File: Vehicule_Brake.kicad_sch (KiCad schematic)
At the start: 22 parts, among them Q51 IRLZ44N, Q53 2N7000, Q54 2N7000, U13 LM339

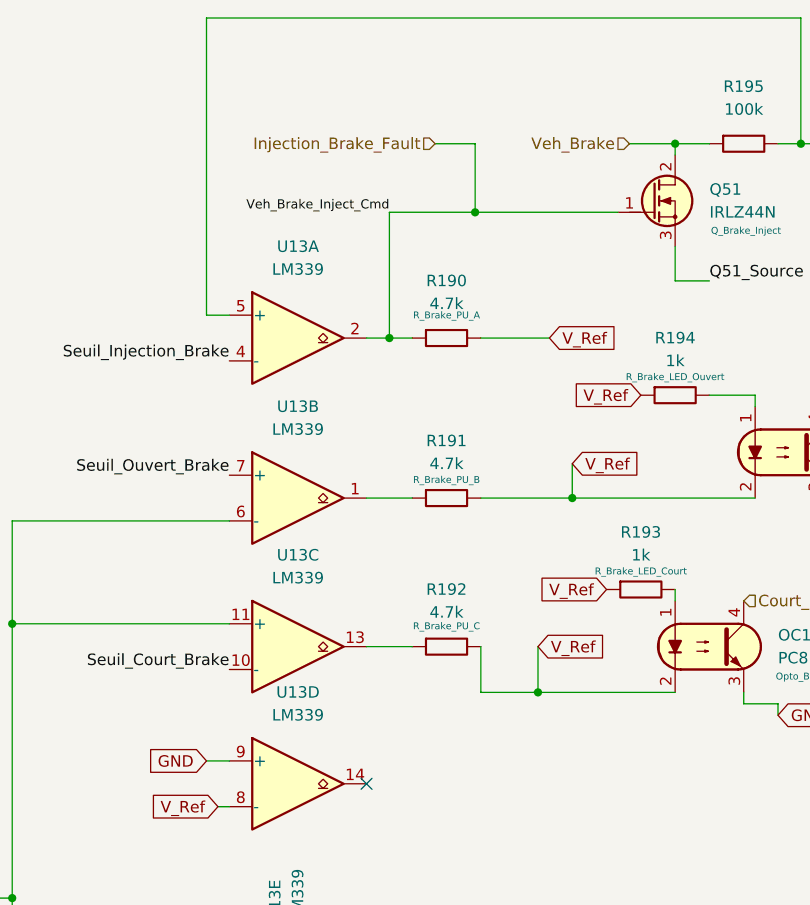
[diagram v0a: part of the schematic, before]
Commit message: Add files via upload
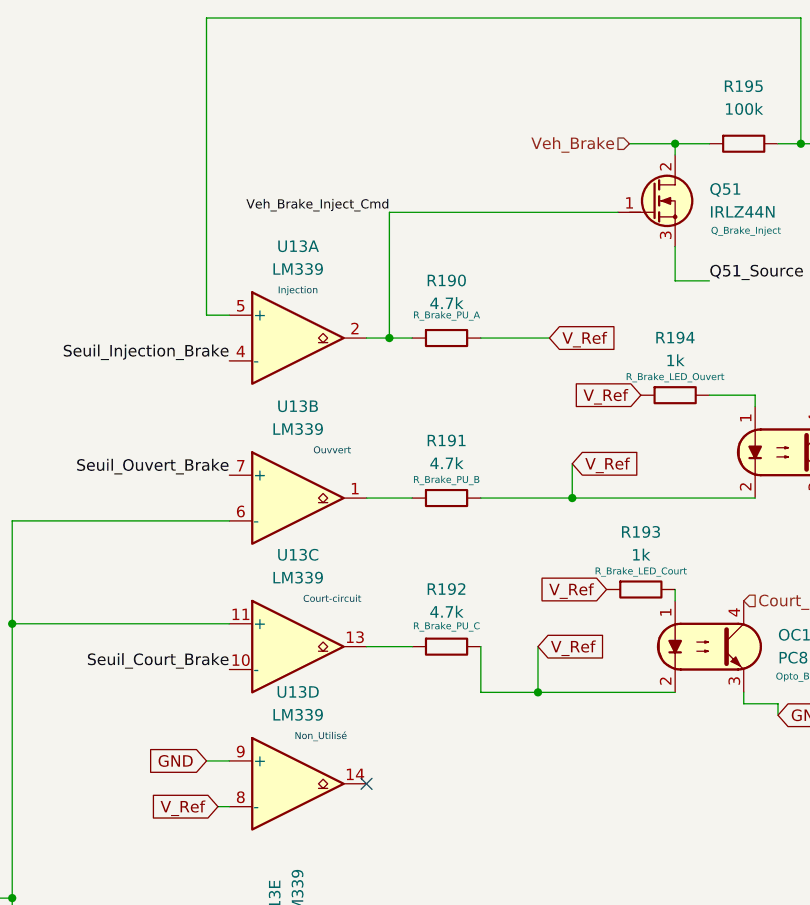
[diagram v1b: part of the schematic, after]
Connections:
- net Injection_Brake_Fault renamed Veh_Brake_Inject_Cmd
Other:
- note added: "Court-circuit"
- note added: "Injection"
- note added: "Non_Utilisé"
- note added: "Ouvvert"
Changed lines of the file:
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@@
+		)
+	)
+	(text "Ouvvert\n"
+		(exclude_from_sim no)
+		(at 83.82 67.31 0)
+		(effects
+			(font
+				(size 0.762 0.762)
+			)
+		)
+	)
+	(text "Court-circuit\n"
+		(exclude_from_sim no)
+		(at 83.82 83.82 0)
+		(effects
+			(font
+				(size 0.762 0.762)
+			)
+		)
+	)
+	(text "Injection"
+		(exclude_from_sim no)
+		(at 80.01 49.53 0)
+		(effects
+			(font
+				(size 0.762 0.762)
+			)
+		)
+	)
+	(text "Non_Utilisé"
+		(exclude_from_sim no)
+		(at 82.55 99.06 0)
+		(effects
+			(font
+				(size 0.762 0.762)
+			)
 		)
 	)
@@
 	)
 	(junction
-		(at 99.695 40.64)
-		(diameter 0)
-		(color 0 0 0 0)
-	)
-	(junction
 		(at 135.89 33.02)
 		(diameter 0)
@@
 	(wire
 		(pts
-			(xy 99.695 33.02) (xy 99.695 40.64)
-		)
-		(stroke
-			(width 0)
-			(type default)
-		)
-	)
-	(wire
-		(pts
 			(xy 212.09 158.75) (xy 212.09 162.56)
 		)
@@
 	(wire
 		(pts
-			(xy 95.25 33.02) (xy 99.695 33.02)
-		)
-		(stroke
-			(width 0)
-			(type default)
-		)
-	)
-	(wire
-		(pts
 			(xy 43.18 127) (xy 48.26 127)
 		)
@@
 	(wire
 		(pts
-			(xy 99.695 40.64) (xy 90.17 40.64)
-		)
-		(stroke
-			(width 0)
-			(type default)
-		)
-	)
-	(wire
-		(pts
 			(xy 48.26 127) (xy 48.26 116.84)
 		)
@@
 	(wire
 		(pts
-			(xy 115.57 40.64) (xy 99.695 40.64)
+			(xy 115.57 40.64) (xy 90.17 40.64)
 		)
 		(stroke
@@
 		)
 	)
-	(hierarchical_label "Injection_Brake_Fault"
-		(shape input)
-		(at 95.25 33.02 180)
-		(effects
-			(font
-				(size 1.27 1.27)
-			)
-			(justify right)
-		)
-	)

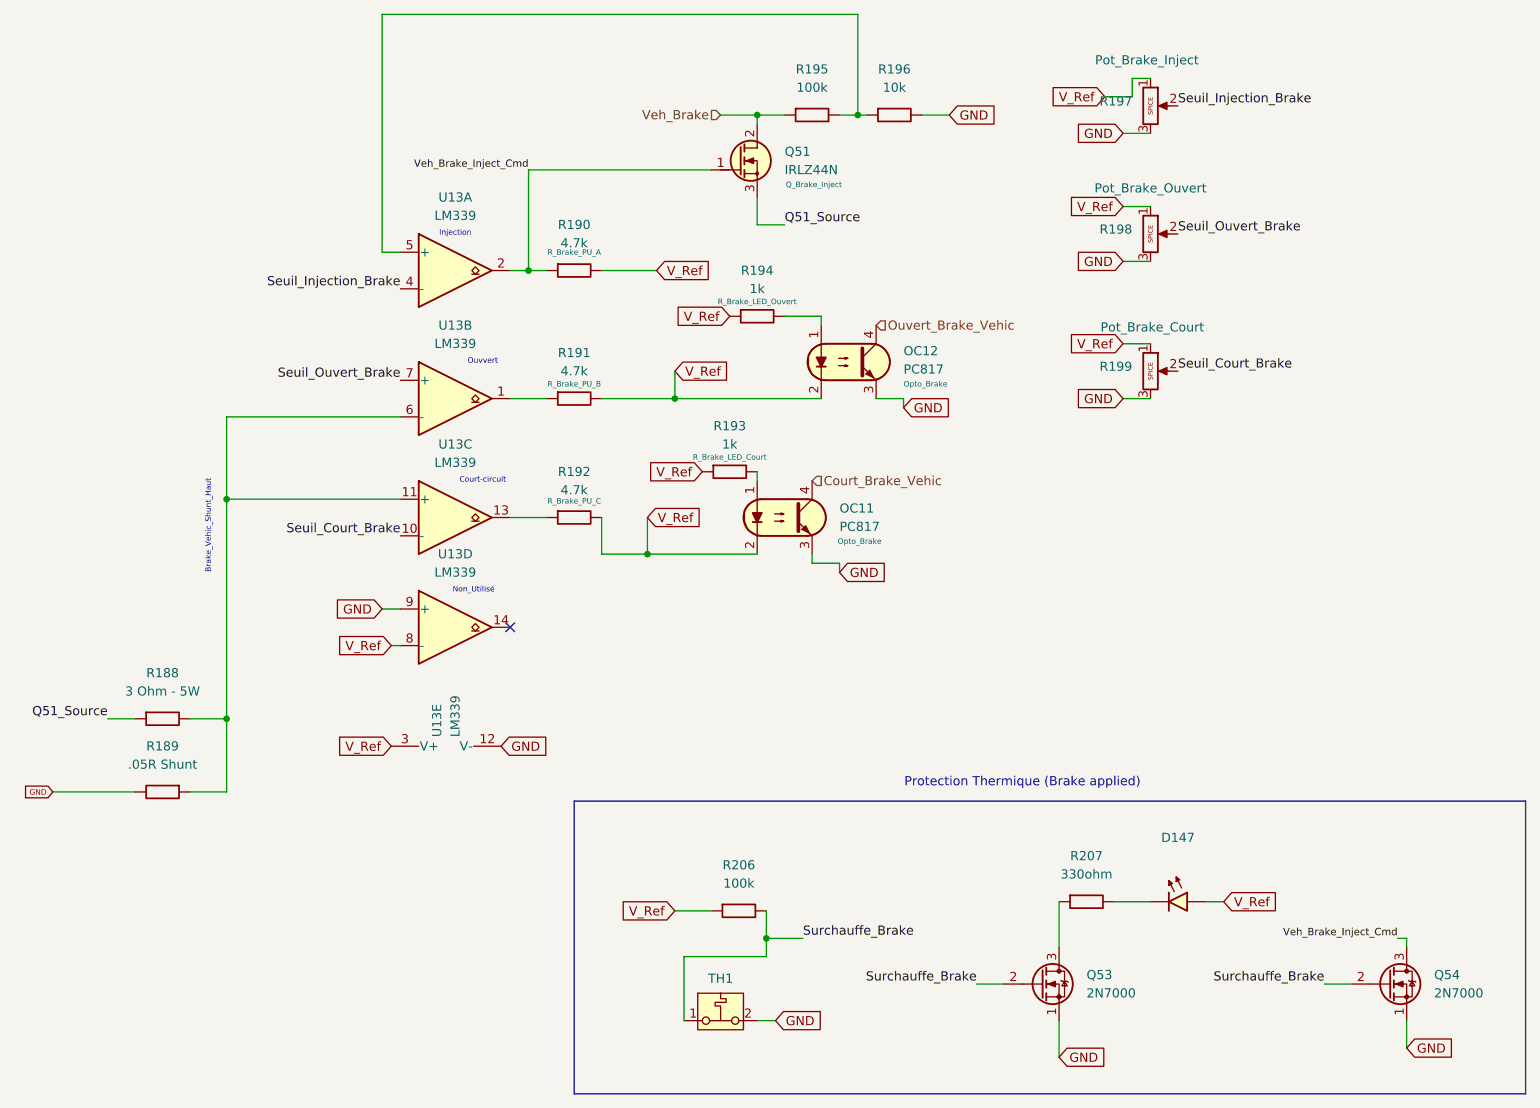
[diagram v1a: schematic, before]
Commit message: Add files via upload
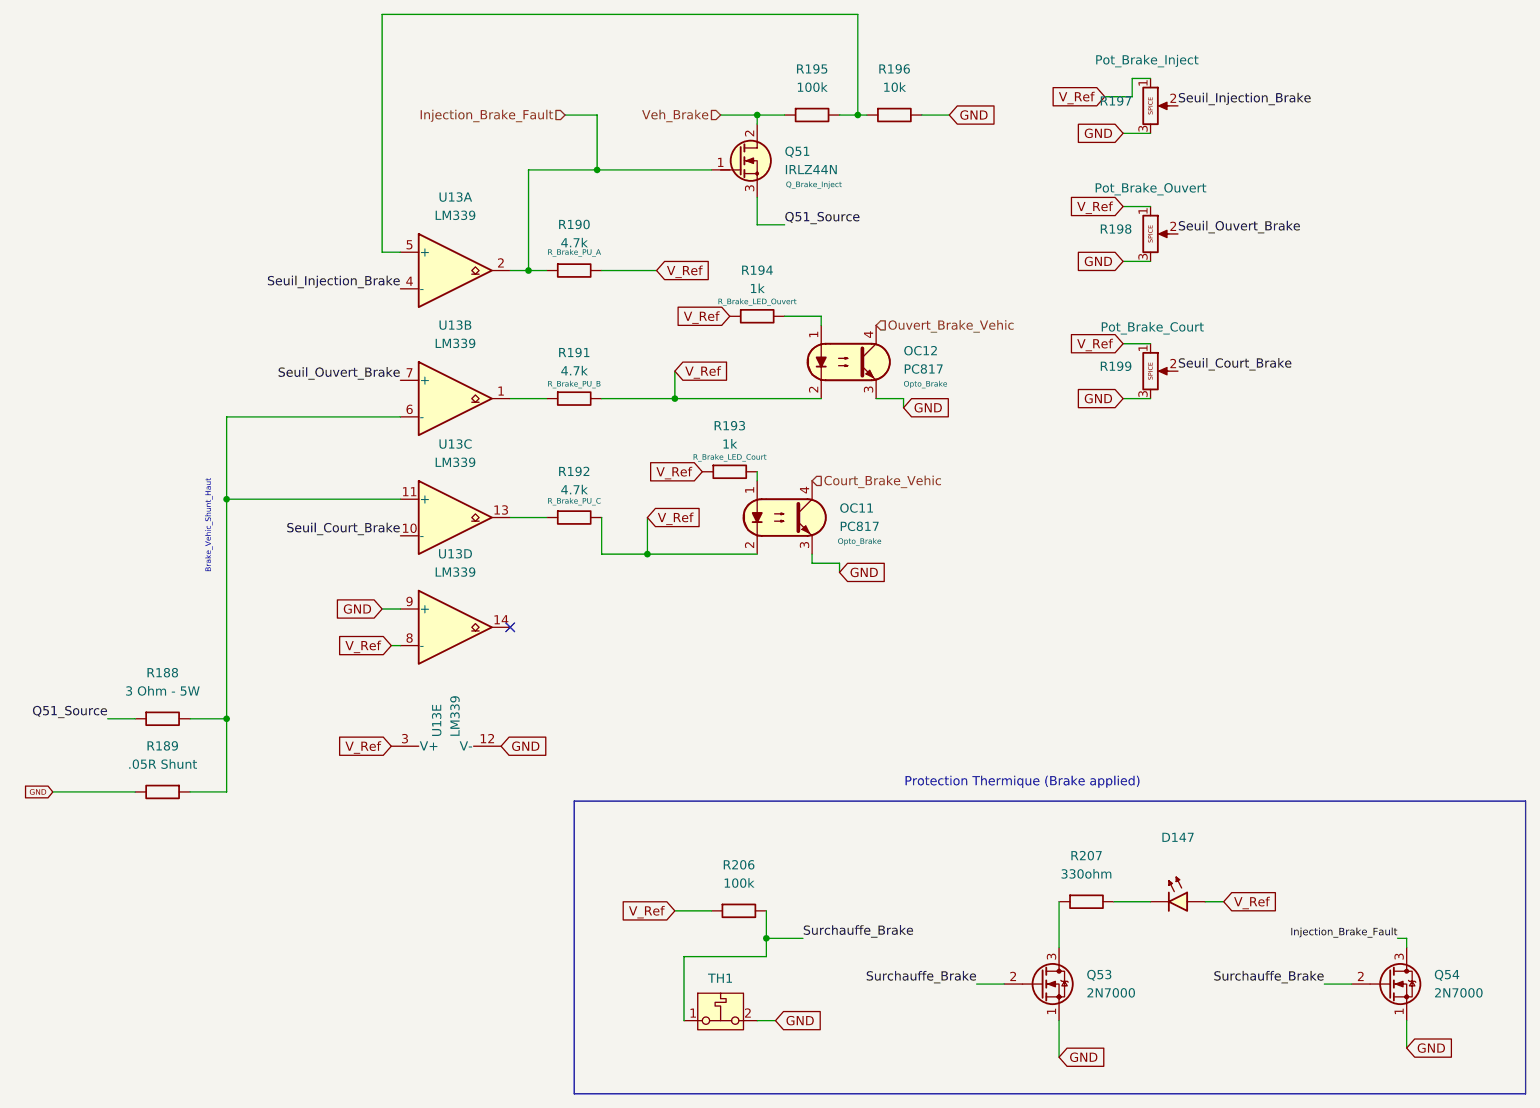
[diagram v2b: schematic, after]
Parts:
- R197, R198, R199: footprint (none) -> TRIM_3296W1103LF:TRIM_3296W1103LF
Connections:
- net Veh_Brake_Inject_Cmd renamed Injection_Brake_Fault
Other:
- note removed: "Court-circuit"
- note removed: "Injection"
- note removed: "Non_Utilisé"
- note removed: "Ouvvert"
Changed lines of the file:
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@@
 		)
 	)
-	(text "Ouvvert\n"
-		(exclude_from_sim no)
-		(at 83.82 67.31 0)
-		(effects
-			(font
-				(size 0.762 0.762)
-			)
-		)
-	)
-	(text "Court-circuit\n"
-		(exclude_from_sim no)
-		(at 83.82 83.82 0)
-		(effects
-			(font
-				(size 0.762 0.762)
-			)
-		)
-	)
-	(text "Injection"
-		(exclude_from_sim no)
-		(at 80.01 49.53 0)
-		(effects
-			(font
-				(size 0.762 0.762)
-			)
-		)
-	)
-	(text "Non_Utilisé"
-		(exclude_from_sim no)
-		(at 82.55 99.06 0)
-		(effects
-			(font
-				(size 0.762 0.762)
-			)
-		)
-	)
 	(text "Brake_Vehic_Shunt_Haut"
 		(exclude_from_sim no)
@@
 	)
 	(junction
+		(at 99.695 40.64)
+		(diameter 0)
+		(color 0 0 0 0)
+	)
+	(junction
 		(at 135.89 33.02)
 		(diameter 0)
@@
 	(wire
 		(pts
+			(xy 99.695 33.02) (xy 99.695 40.64)
+		)
+		(stroke
+			(width 0)
+			(type default)
+		)
+	)
+	(wire
+		(pts
 			(xy 212.09 158.75) (xy 212.09 162.56)
 		)
@@
 	(wire
 		(pts
+			(xy 95.25 33.02) (xy 99.695 33.02)
+		)
+		(stroke
+			(width 0)
+			(type default)
+		)
+	)
+	(wire
+		(pts
 			(xy 43.18 127) (xy 48.26 127)
 		)
@@
 	(wire
 		(pts
+			(xy 99.695 40.64) (xy 90.17 40.64)
+		)
+		(stroke
+			(width 0)
+			(type default)
+		)
+	)
+	(wire
+		(pts
 			(xy 48.26 127) (xy 48.26 116.84)
 		)
@@
 	(wire
 		(pts
-			(xy 115.57 40.64) (xy 90.17 40.64)
+			(xy 115.57 40.64) (xy 99.695 40.64)
 		)
 		(stroke
@@
 		)
 	)
-	(label "Veh_Brake_Inject_Cmd"
-		(at 90.17 40.64 180)
-		(effects
-			(font
-				(size 1.016 1.016)
-			)
-			(justify right bottom)
-		)
-	)
 	(label "Surchauffe_Brake"
 		(at 152.4 153.67 180)
@@
 		)
 	)
-	(label "Veh_Brake_Inject_Cmd"
+	(label "Injection_Brake_Fault"
 		(at 210.82 147.32 180)
 		(effects
@@
 		)
 	)
+	(hierarchical_label "Injection_Brake_Fault"
+		(shape input)
+		(at 95.25 33.02 180)
+		(effects
+			(font
+				(size 1.27 1.27)
+			)
+			(justify right)
+		)
+	)
 	(hierarchical_label "Veh_Brake"
 		(shape input)
@@
 			)
 		)
-		(property "Footprint" ""
+		(property "Footprint" "TRIM_3296W1103LF:TRIM_3296W1103LF"
 			(at 176.53 49.53 0)
 			(hide yes)
@@
 			)
 		)
-		(property "Footprint" ""
+		(property "Footprint" "TRIM_3296W1103LF:TRIM_3296W1103LF"
 			(at 176.53 31.75 0)
 			(hide yes)
@@
 			)
 		)
-		(property "Footprint" ""
+		(property "Footprint" "TRIM_3296W1103LF:TRIM_3296W1103LF"
 			(at 176.53 68.58 0)
 			(hide yes)

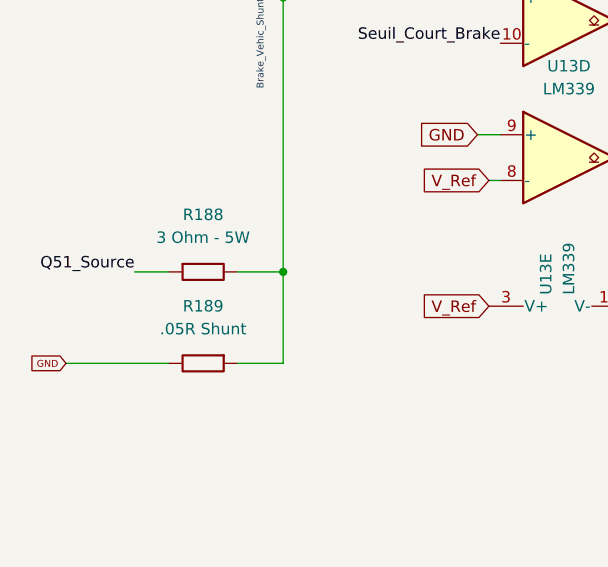
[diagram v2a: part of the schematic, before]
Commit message: Add files via upload
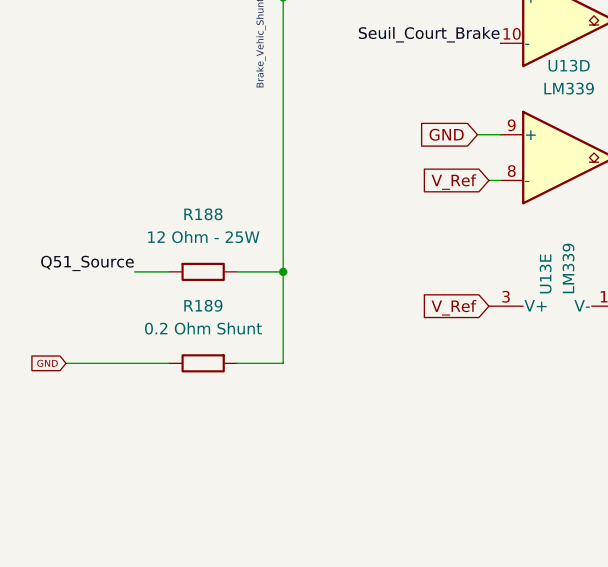
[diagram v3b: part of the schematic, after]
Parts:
- R188: value 3 Ohm - 5W -> 12 Ohm - 25W; footprint Resistor_THT:R_Axial_Power_L25.0mm_W9.0mm_P27.94mm -> TerminalBlock_Phoenix:TerminalBlock_Phoenix_PT-1,5-2-3.5-H_1x02_P3.50mm_Horizontal
- R189: value .05R Shunt -> 0.2 Ohm Shunt
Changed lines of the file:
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@@
 			)
 		)
-		(property "Value" "3 Ohm - 5W"
+		(property "Value" "12 Ohm - 25W"
 			(at 39.37 113.03 0)
 			(show_name no)
@@
 			)
 		)
-		(property "Footprint" "Resistor_THT:R_Axial_Power_L25.0mm_W9.0mm_P27.94mm"
+		(property "Footprint" "TerminalBlock_Phoenix:TerminalBlock_Phoenix_PT-1,5-2-3.5-H_1x02_P3.50mm_Horizontal"
 			(at 40.259 121.158 0)
 			(hide yes)
@@
 			)
 		)
-		(property "Description" "5W Resistor"
+		(property "Description" "25W Resistor"
 			(at 39.37 116.84 0)
 			(hide yes)
@@
 			)
 		)
-		(property "Value" ".05R Shunt"
+		(property "Value" "0.2 Ohm Shunt"
 			(at 39.37 123.19 0)
 			(show_name no)
